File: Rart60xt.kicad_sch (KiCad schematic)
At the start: 8 parts, among them Y1 12MHz

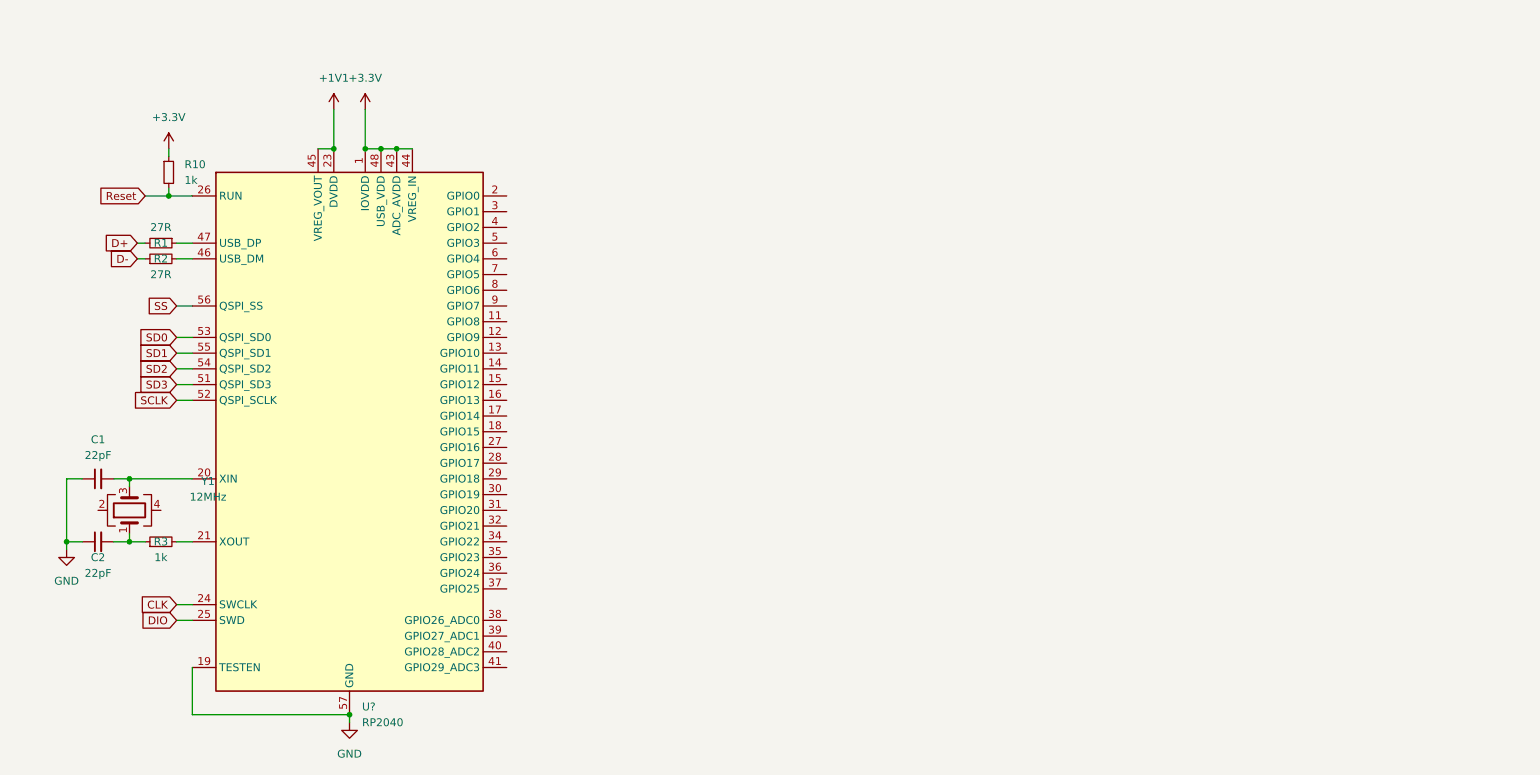
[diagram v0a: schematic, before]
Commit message: Process
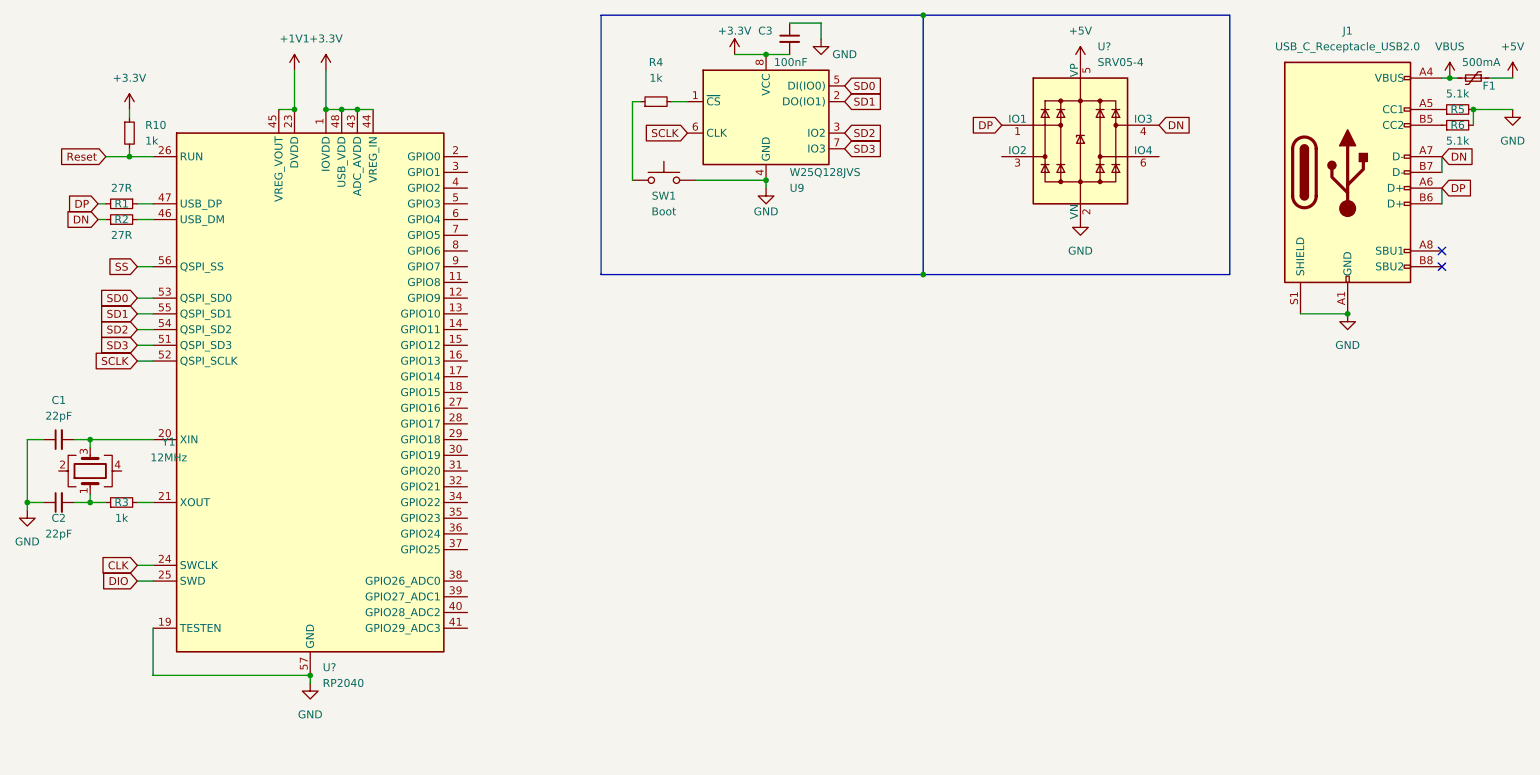
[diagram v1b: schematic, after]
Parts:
- added C3: 100nF, symbol Device:C_Small
- added F1: 500mA, symbol Device:Polyfuse_Small
- added J1: USB_C_Receptacle_USB2.0, symbol Connector:USB_C_Receptacle_USB2.0
- added R4: 1k, symbol Device:R_Small
- added R5, R6: 5.1k, symbol Device:R_Small
- added SW1: Boot, symbol Switch:SW_Push
- added U9: W25Q128JVS, Package_SO:SOIC-8_5.23x5.23mm_P1.27mm, symbol Memory_Flash:W25Q128JVS
- added U?: SRV05-4, Package_TO_SOT_SMD:SOT-23-6, symbol Power_Protection:SRV05-4
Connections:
- net +3.3V: now also C3.2, U9.8 (VCC)
- net GND: now also C3.1, J1.A1 (GND), J1.A12 (GND), J1.B1 (GND), J1.B12 (GND), J1.S1 (SHIELD), R5.2, R6.2, SW1.2, U9.4 (GND), U?.2 (VN)
- net SCLK: now also U9.6 (CLK)
- net SD0: now also U9.5 (DI(IO0))
- net SD1: now also U9.2 (DO(IO1))
- net SD2: now also U9.3 (IO2)
- net SD3: now also U9.7 (IO3)
- net D+ renamed DP
- net DP: now also J1.A6 (D+), J1.B6 (D+), U?.1 (IO1)
- net D- renamed DN
- net DN: now also J1.A7 (D-), J1.B7 (D-), U?.4 (IO3)
- new net: J1.B5 (CC2), R6.1
- new net: R4.1, SW1.1
- new net: J1.A5 (CC1), R5.1
- new net: R4.2, U9.1 (~{CS})
- new net +5V: F1.1, U?.5 (VP)
- new net VBUS: F1.2, J1.A4 (VBUS), J1.A9 (VBUS), J1.B4 (VBUS), J1.B9 (VBUS)
- no-connect marks 0 -> 2
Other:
- moved on the sheet: C1, C2, R1, R10, R2, R3, U?, Y1
